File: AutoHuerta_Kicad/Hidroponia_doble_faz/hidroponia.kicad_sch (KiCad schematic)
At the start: 37 parts, among them J1 bornera, J2 bornera, J3 Barrel_Jack, J4 pin, J6 Pin, J7 Pin, K1 RELAY, Q1 BC817, Q2 BS170F, Q3 BC817, U2 PC817, U3 L7805, U4 PC817, U5 L7805, U6 PC817

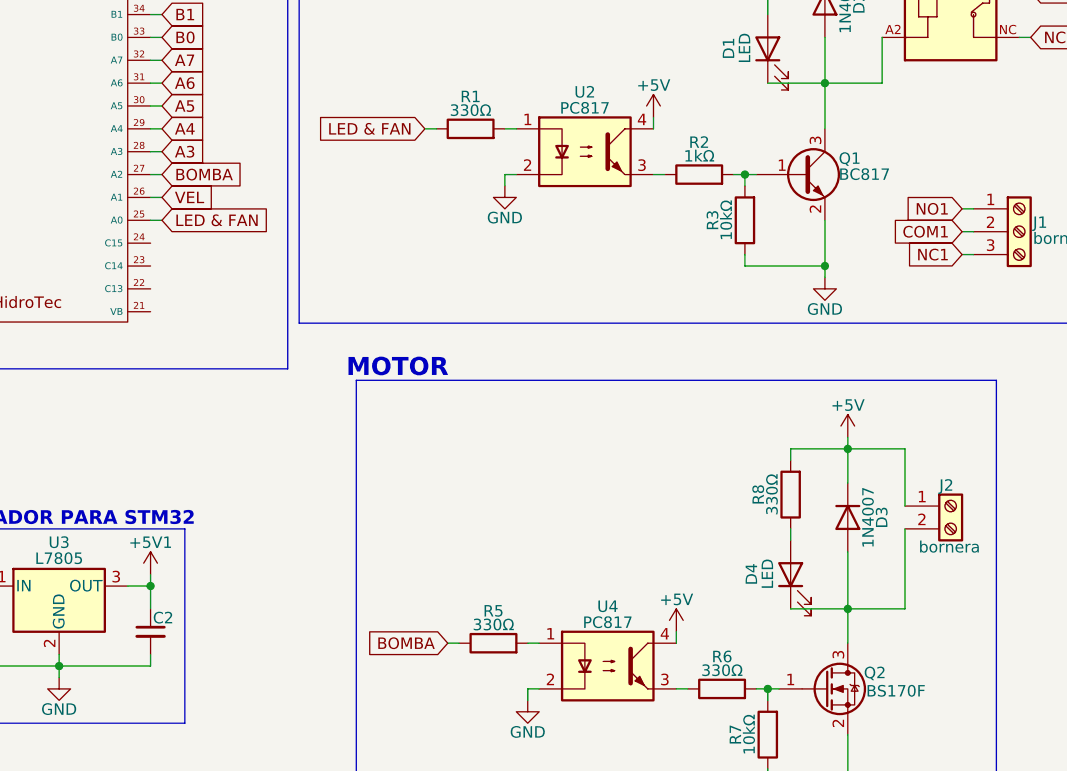
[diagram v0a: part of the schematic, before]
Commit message: PCB TERMINADO
Terminamos el PCB
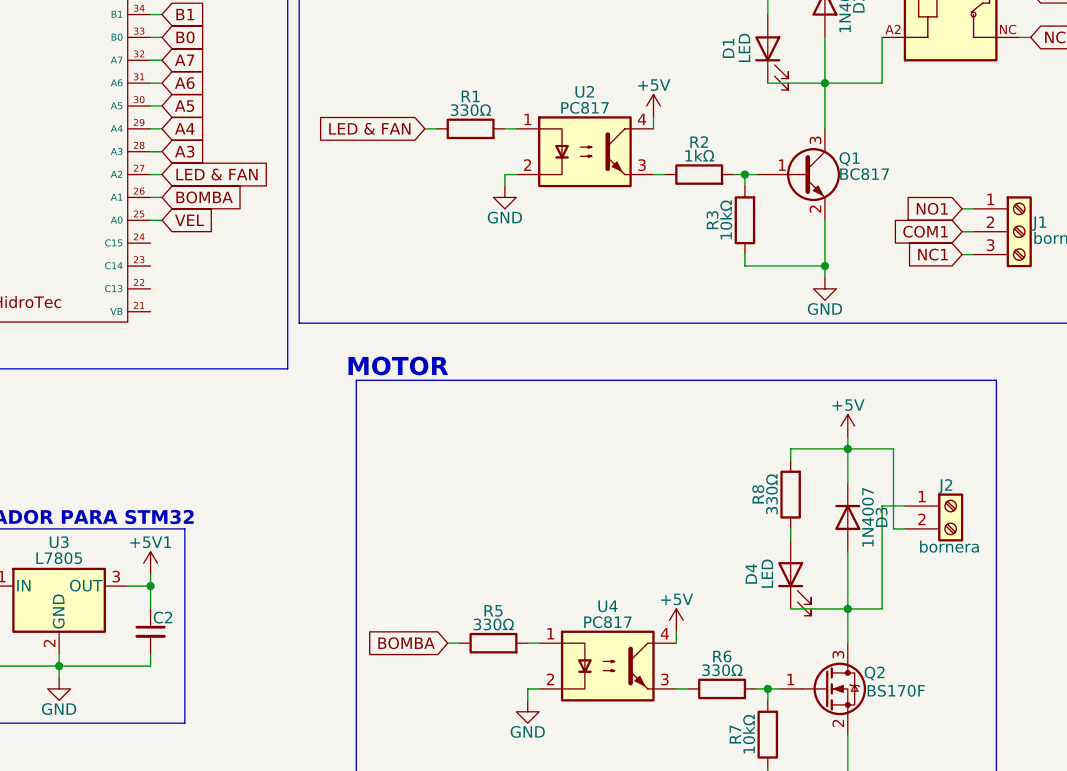
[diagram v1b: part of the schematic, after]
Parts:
- C1: footprint Capacitor_SMD:C_0805_2012Metric_Pad1.18x1.45mm_HandSolder -> Capacitor_SMD:C_0504_1310Metric_Pad0.83x1.28mm_HandSolder
- J2: footprint TerminalBlock_MetzConnect:TerminalBlock_MetzConnect_Type011_RT05502HBWC_1x02_P5.00mm_Horizontal -> TerminalBlock:TerminalBlock_bornier-2_P5.08mm
- U5: footprint Package_TO_SOT_SMD:TO-252-2 -> Package_TO_SOT_SMD:TO-263-2_TabPin1
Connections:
- net +5V: now also J2.2 (Pin_2); no longer J2.1 (Pin_1)
- net BOMBA: now also U1.26 (A1); no longer U1.27 (A2)
- net LED & FAN: now also U1.27 (A2); no longer U1.25 (A0)
- net VEL: now also U1.25 (A0); no longer U1.26 (A1)
- net at D3.2 (A), D4.1 (K), Q2.3 (D): now also J2.1 (Pin_1); no longer J2.2 (Pin_2)
